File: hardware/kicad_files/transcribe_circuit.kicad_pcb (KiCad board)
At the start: 2 copper layers, 100 x 45 mm, 23 parts, among them J1 europower, J2 RS232_SERIAL, J3 RS232_DSUB, J4 MIDI_IN_TRS, J5 MIDI_IN_DIN, J6 MIDI_OUT_TRS, J7 MIDI_OUT_DIN, U1 ProMicro, U2 MAX232, U3 6N137, U4 4069, U5 usbHostMini, U6 L78L33_TO92

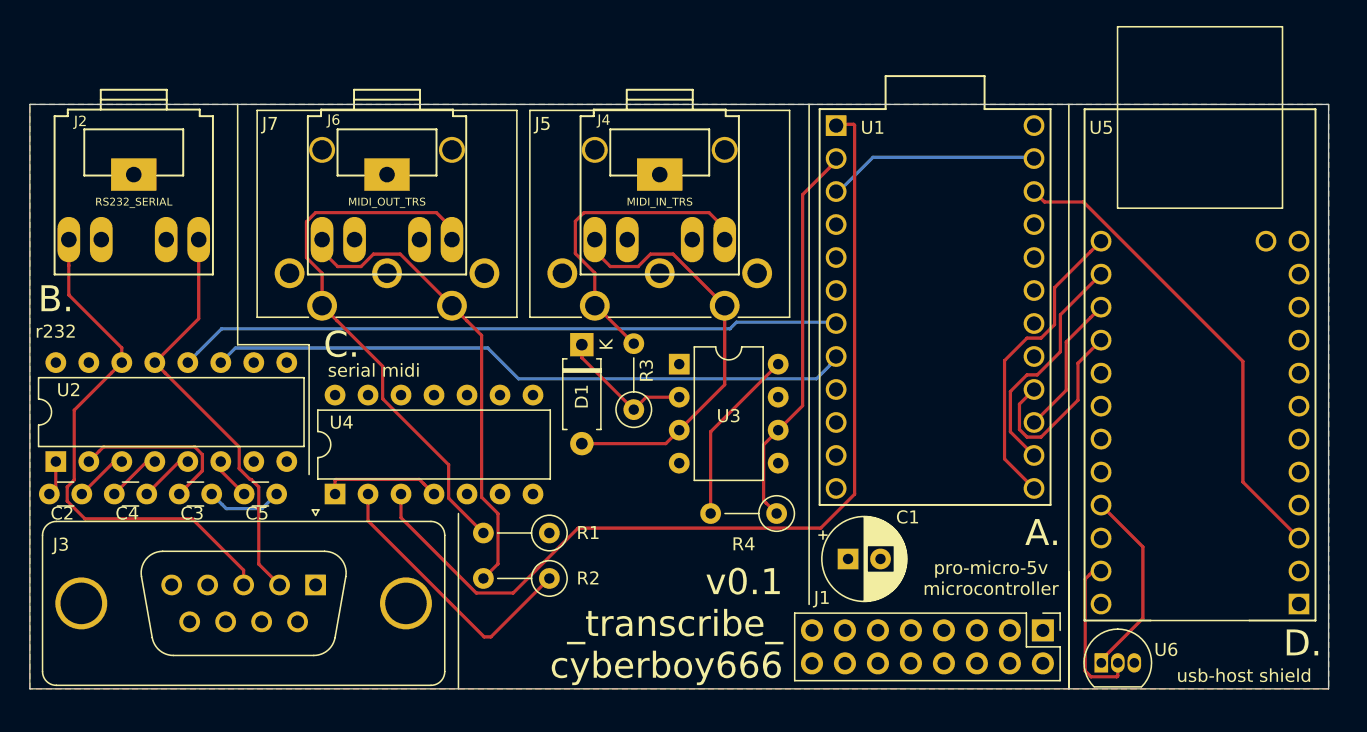
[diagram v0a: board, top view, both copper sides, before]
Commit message: small pcb fixes
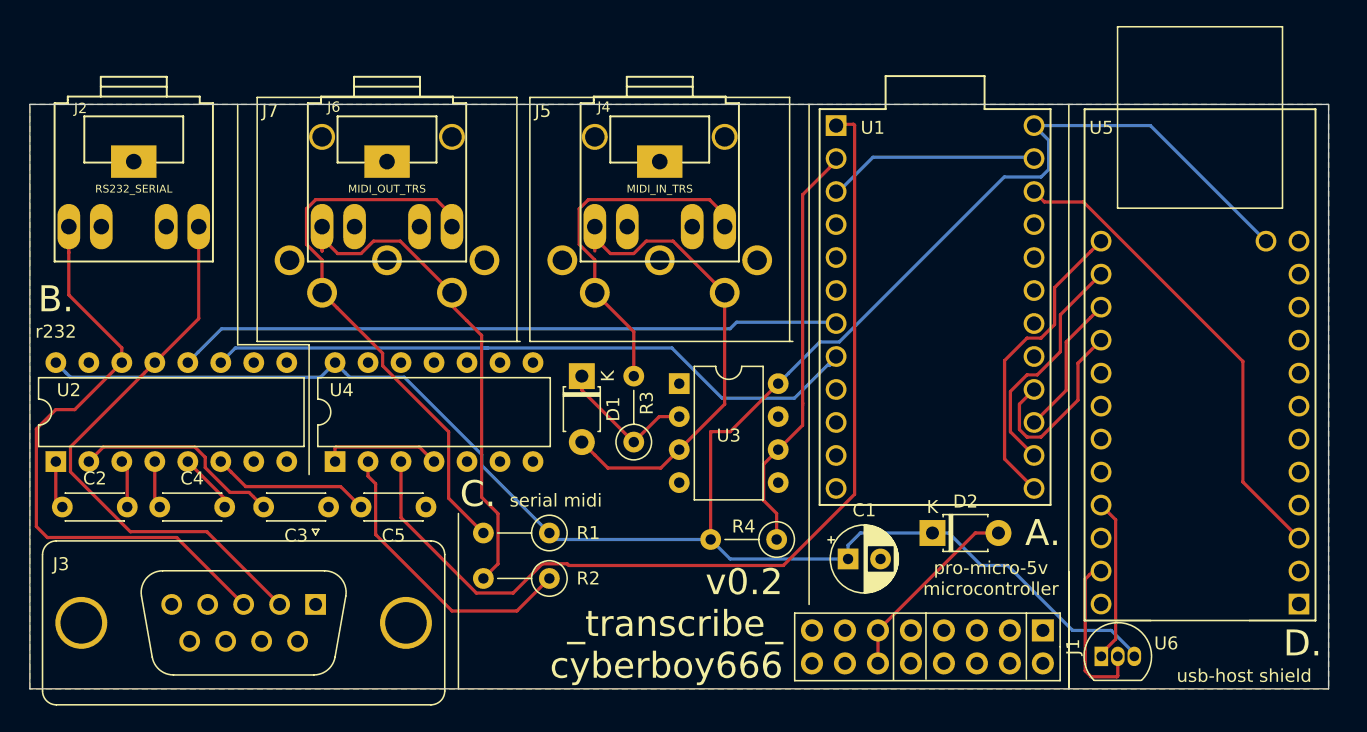
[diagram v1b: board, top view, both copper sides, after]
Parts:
- added D2: 1N4148, Diode_THT:D_T-1_P5.08mm_Horizontal, F.Cu at (-220.5, -757.0)
- C1: footprint Capacitor_THT:CP_Radial_D6.3mm_P2.50mm -> Capacitor_THT:CP_Radial_D5.0mm_P2.50mm
- C2, C3, C4, C5: footprint Capacitor_THT:C_Disc_D3.0mm_W1.6mm_P2.50mm -> Capacitor_THT:C_Disc_D4.3mm_W1.9mm_P5.00mm
- D1: footprint Diode_THT:D_A-405_P7.62mm_Horizontal -> Diode_THT:D_T-1_P5.08mm_Horizontal
- J1: footprint Connector_PinHeader_2.54mm:PinHeader_2x08_P2.54mm_Vertical -> lib_fp:PinHeader_2x08_P2.54_Euro
- J2, J4, J6: footprint Connector_Audio:Tayda_3.5mm_stereo_TRS_jack_A-853 -> lib_fp:Tayda_3.5mm_stereo_TRS_jack_A-853
- J5, J7: footprint Connector_DIN:Tayda5pinMidi-A1010 -> lib_fp:Tayda5pinMidi-A1010
- moved C5 11.5 mm to (-259.5, -759.0)
- moved C3 9.06 mm to (-267.0, -759.0)
- moved C4 3.64 mm to (-280.0, -759.0)
- moved R3 2.50 mm to (-243.5, -764.0)
- moved U4 2.50 mm to (-266.5, -762.5)
- moved D1 2.42 mm to (-247.5, -769.1)
- moved R4 2.00 mm to (-232.5, -756.5)
- moved J3 1.50 mm to (-268.0, -751.5)
- moved U3 1.50 mm to (-240.0, -768.5)
- moved C2 1.41 mm to (-287.5, -759.0)
- moved J2 1.00 mm to (-282.0, -784.0)
- moved J4 1.00 mm to (-241.5, -784.0)
- moved J5 1.00 mm to (-249.0, -778.0)
- moved J6 1.00 mm to (-262.5, -784.0)
- moved J7 1.00 mm to (-270.0, -778.0)
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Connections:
- J1 pad 11: +5V -> Net-(D2-Pad2)
- J1 pad 12: +5V -> Net-(D2-Pad2)
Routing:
- net +5V: track 13.7 -> 164.3 mm
- net Net-(D2-Pad2): track 0.00 -> 14.9 mm
- net RS_SERIAL_IN: track 32.0 -> 43.3 mm
- net Net-(C5-Pad2): track 3.25 -> 12.9 mm
- net RS_SERIAL_OUT: track 40.5 -> 46.8 mm
- net GND: track 34.6 -> 28.7 mm
- net MIDI_IN_PLUS: track 24.5 -> 28.5 mm
- net MIDI_IN_DATA: track 32.4 -> 35.7 mm
- net Net-(C3-Pad2): track 13.2 -> 16.3 mm
- net MIDI_OUT_DATA: track 36.4 -> 39.1 mm
- net MIDI_SERIAL_OUT: track 71.9 -> 74.5 mm
- net ALT_SERIAL_OUT: track 49.9 -> 52.4 mm
- net 3.3v: track 14.8 -> 12.6 mm
- net MIDI_SERIAL_IN: track 30.3 -> 32.5 mm
- net MIDI_OUT_PLUS: track 42.5 -> 44.3 mm
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- added copper zone on B.Cu, net GND
- removed copper zone on B.Cu, net +5V
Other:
- board text added: "v0.2 _transcribe_ cyberboy666"
- board text removed: "v0.1 _transcribe_ cyberboy666"
